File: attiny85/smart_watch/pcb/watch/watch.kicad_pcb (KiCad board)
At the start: 2 copper layers, 5 parts, among them J1 Conn_01x04_Pin, SW1 Wake, SW2 Select, SW3 Set, U1 ATTINY85

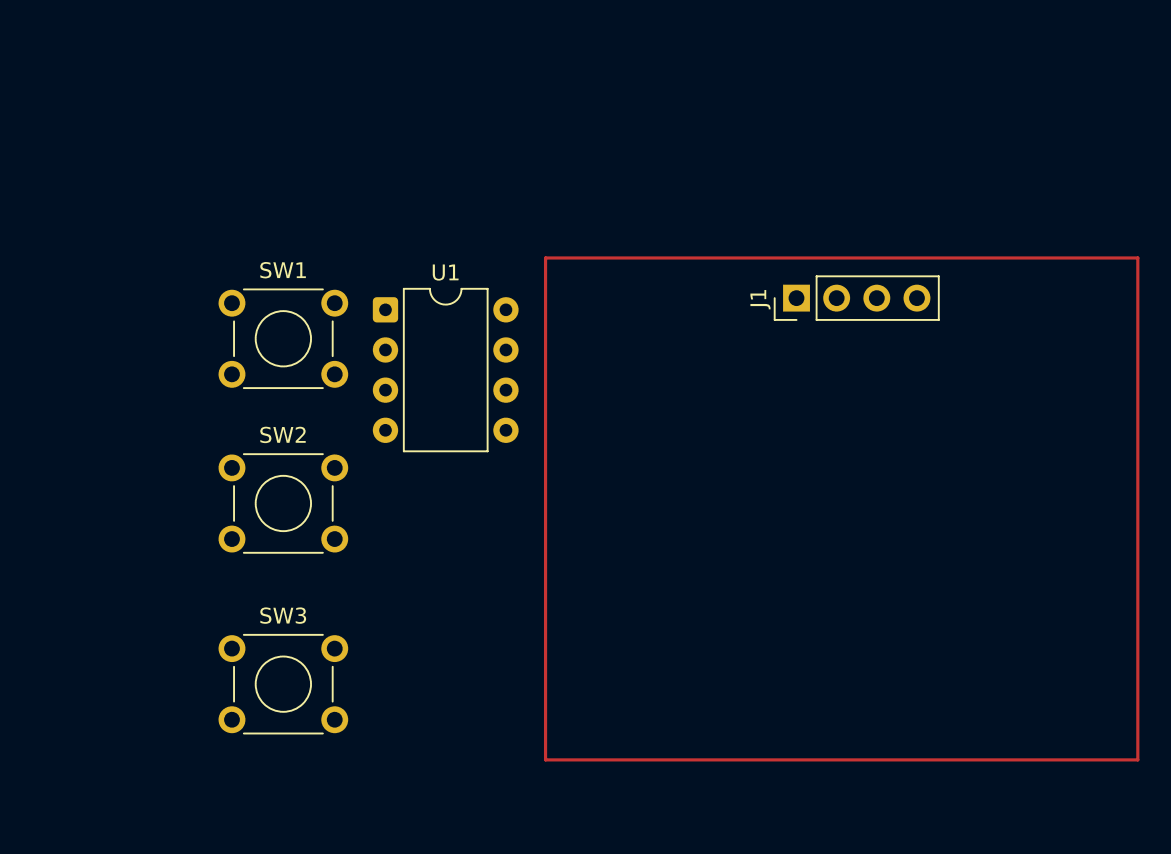
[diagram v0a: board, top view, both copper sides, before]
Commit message: PCB mounting
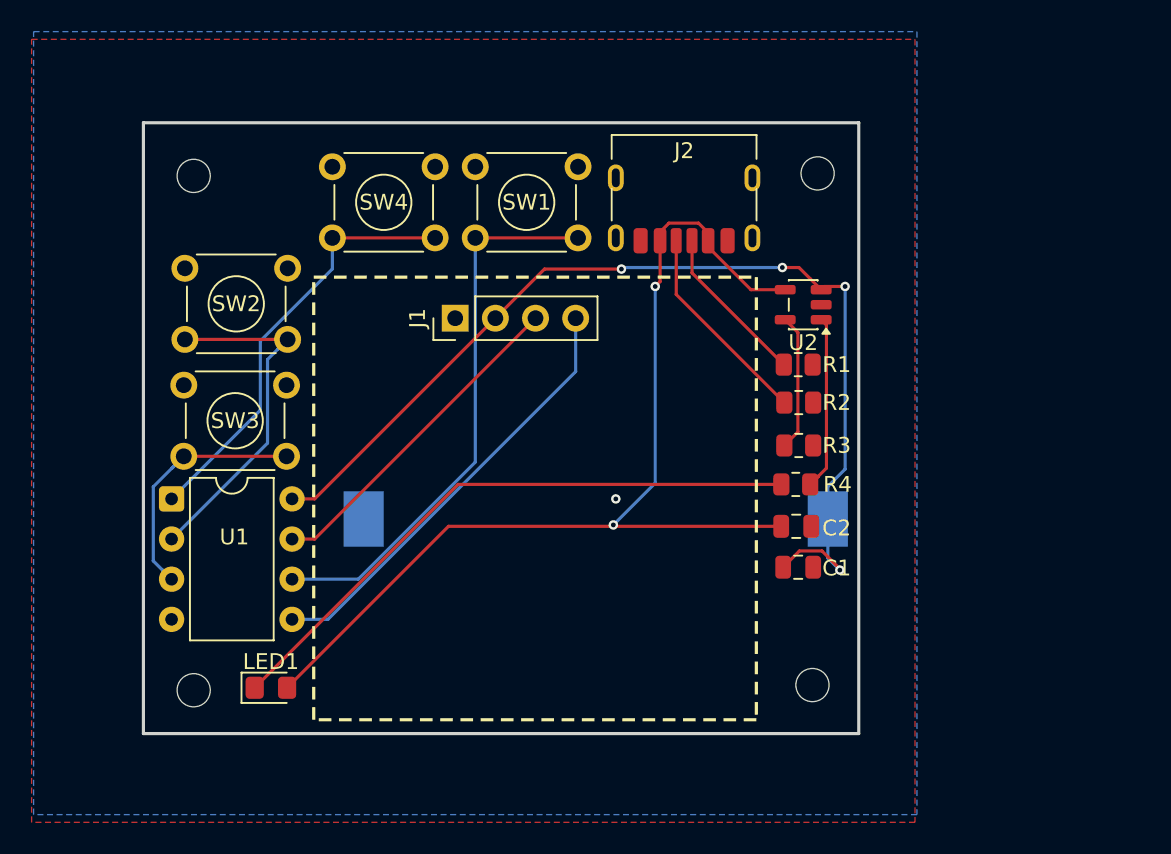
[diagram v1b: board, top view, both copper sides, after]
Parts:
- added BT1: Battery_Cell, Battery:BatteryHolder_Keystone_1058_1x2032, B.Cu at (151.1, 90.2)
- added C1: 4.7uF, Capacitor_SMD:C_0805_2012Metric, F.Cu at (163.9, 93.2)
- added C2: 4.7uF, Capacitor_SMD:C_0805_2012Metric, F.Cu at (163.8, 90.6)
- added H1: MountingHole, MountingHole:MountingHole_2.1mm, F.Cu at (125.7, 68.5)
- added H2: MountingHole, MountingHole:MountingHole_2.1mm, F.Cu at (125.7, 101.0)
- added H3: MountingHole, MountingHole:MountingHole_2.1mm, F.Cu at (164.8, 100.7)
- added H4: MountingHole, MountingHole:MountingHole_2.1mm, F.Cu at (165.2, 68.3)
- added J2: USB C, Connector_USB:USB_C_Receptacle_HRO_TYPE-C-31-M-17, F.Cu at (156.7, 69.4)
- added LED1: Charger LED, LED_SMD:LED_0805_2012Metric_Pad1.15x1.40mm_HandSolder, F.Cu at (130.6, 100.8)
- added R1: 5.1k, Resistor_SMD:R_0805_2012Metric, F.Cu at (163.9, 80.4)
- added R2: 5.1k, Resistor_SMD:R_0805_2012Metric, F.Cu at (164.0, 82.8)
- added R3: 3.6k, Resistor_SMD:R_0805_2012Metric, F.Cu at (164.0, 85.5)
- added R4: 470, Resistor_SMD:R_0805_2012Metric, F.Cu at (163.8, 88.0)
- added SW4: Reset, Button_Switch_THT:SW_TH_Tactile_Omron_B3F-100x, F.Cu at (134.5, 67.9)
- added U2: MCP73831-2-OT, Package_TO_SOT_SMD:SOT-23-5, F.Cu at (164.3, 76.6)
- J1: value Conn_01x04_Pin -> Display
- moved J1 21.6 mm to (142.2, 77.5)
- moved U1 18.1 mm to (124.3, 88.9)
- moved SW1 17.6 mm to (143.5, 67.9)
- moved SW3 16.9 mm to (125.1, 81.7)
- moved SW2 13.0 mm to (125.1, 74.3)
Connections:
- net Select renamed SELECT
- net Set renamed SET
- net Wake renamed WAKE
- U1 pad 1: unconnected-(U1-~{RESET}/PB5-Pad1) -> RESET
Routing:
- net VBUS: track 0.00 -> 65.7 mm, vias 0 -> 2
- net VCC: track 0.00 -> 65.0 mm, vias 0 -> 4
- net Net-(LED1-K): track 0.00 -> 38.6 mm
- net WAKE: track 0.00 -> 35.3 mm
- net SDA: track 0.00 -> 27.8 mm
- net RESET: track 0.00 -> 27.2 mm
- net SELECT: track 0.00 -> 23.1 mm
- net SCK: track 0.00 -> 21.2 mm
- net SET: track 0.00 -> 17.5 mm
- net Net-(J2-CC2): track 0.00 -> 13.1 mm
- net Net-(U2-STAT): track 0.00 -> 11.7 mm
- net Net-(J2-CC1): track 0.00 -> 10.2 mm
- net Net-(U2-PROG): track 0.00 -> 8.64 mm
- net GND: vias 0 -> 1
- added copper zone on B.Cu, net GND
- added copper zone on F.Cu, net GND
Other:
- board outline added: 45.2 x 38.6 mm

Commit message: production files
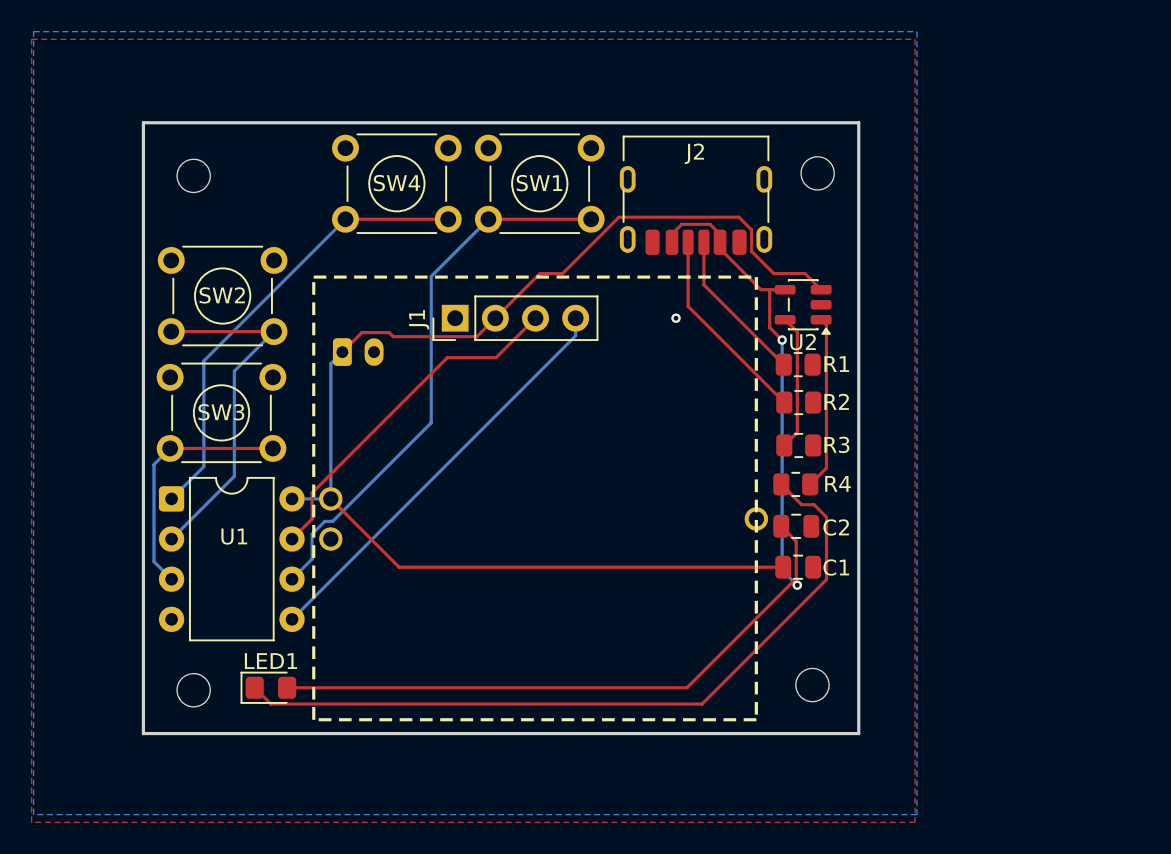
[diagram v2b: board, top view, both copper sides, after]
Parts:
- added J3: LiPo Batt, Connector_JST:JST_PH_S2B-PH-K_1x02_P2.00mm_Horizontal, B.Cu at (135.1, 79.6)
- BT1: value Battery_Cell -> 1059; footprint Battery:BatteryHolder_Keystone_1058_1x2032 -> BatteryHolder_Keystone_1059_THT:BatteryHolder_Keystone_1059_THT
- moved BT1 3.30 mm to (147.8, 90.2)
- moved SW1 1.44 mm to (144.3, 66.7)
- moved SW4 1.44 mm to (135.3, 66.7)
- moved SW3 0.99 mm to (124.2, 81.2)
- moved SW2 0.99 mm to (124.3, 73.8)
- moved J2 0.76 mm to (157.5, 69.5)
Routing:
- net VCC: track 65.0 -> 79.2 mm, vias 4 -> 0
- net Net-(LED1-K): track 38.6 -> 47.5 mm
- net VBUS: track 65.7 -> 68.7 mm
- net SET: track 17.5 -> 15.7 mm
- net RESET: track 27.2 -> 28.7 mm
- net SDA: track 27.8 -> 26.5 mm
- net SCK: track 21.2 -> 22.2 mm
- net SELECT: track 23.1 -> 22.3 mm
- net Net-(U2-STAT): track 11.7 -> 11.0 mm
- net WAKE: track 35.3 -> 34.7 mm
